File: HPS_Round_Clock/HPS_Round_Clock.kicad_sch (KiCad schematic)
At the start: 113 parts, among them J1 PJ-102AH, J2 Conn_01x06, SW1 Omron_B3F_SPST, SW2 Omron_B3F_SPST, SW3 Omron_B3F_SPST, SW4 Omron_B3F_SPST, SW5 Omron_B3F_SPST, U1 L7805, U2 DS1307_DIP-8, U3 MAX7219, U4 ATmega328-PU, U5 TSOP38238, Y1 Crystal_16MHz, Y2 Crystal_32768Hz

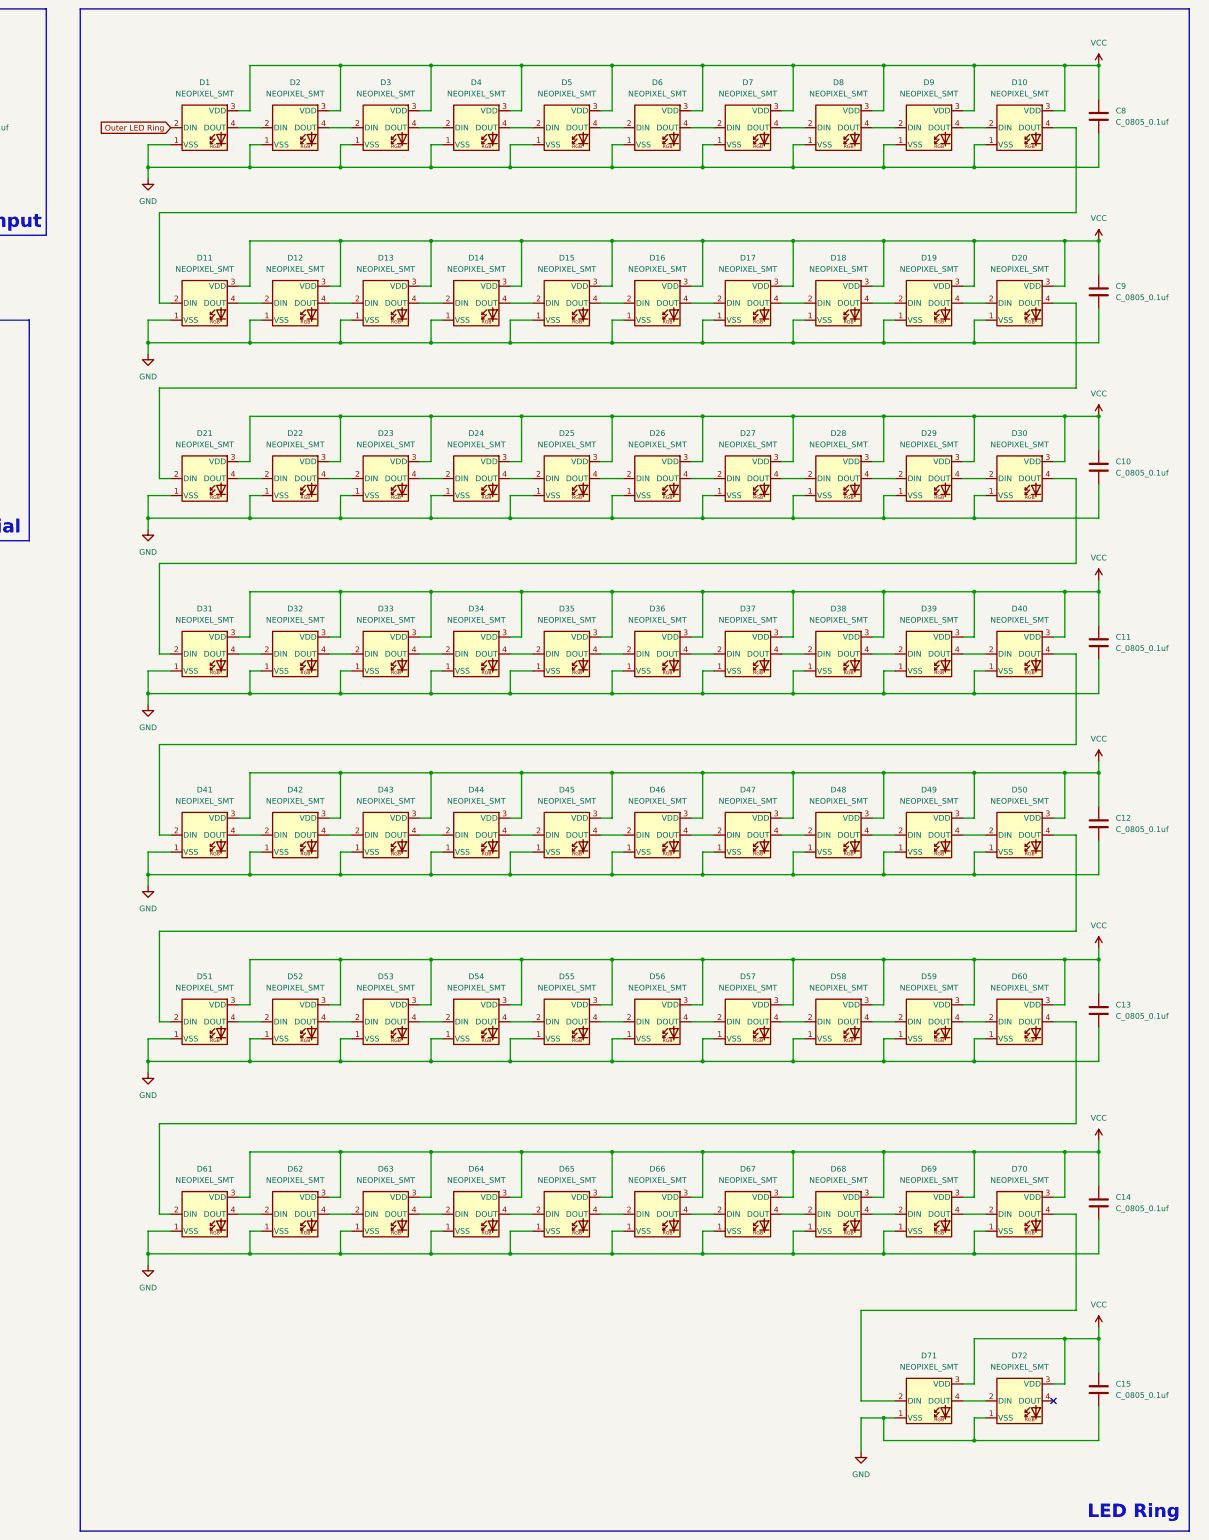
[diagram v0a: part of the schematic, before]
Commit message: Update HPS_Round_Clock.kicad_sch
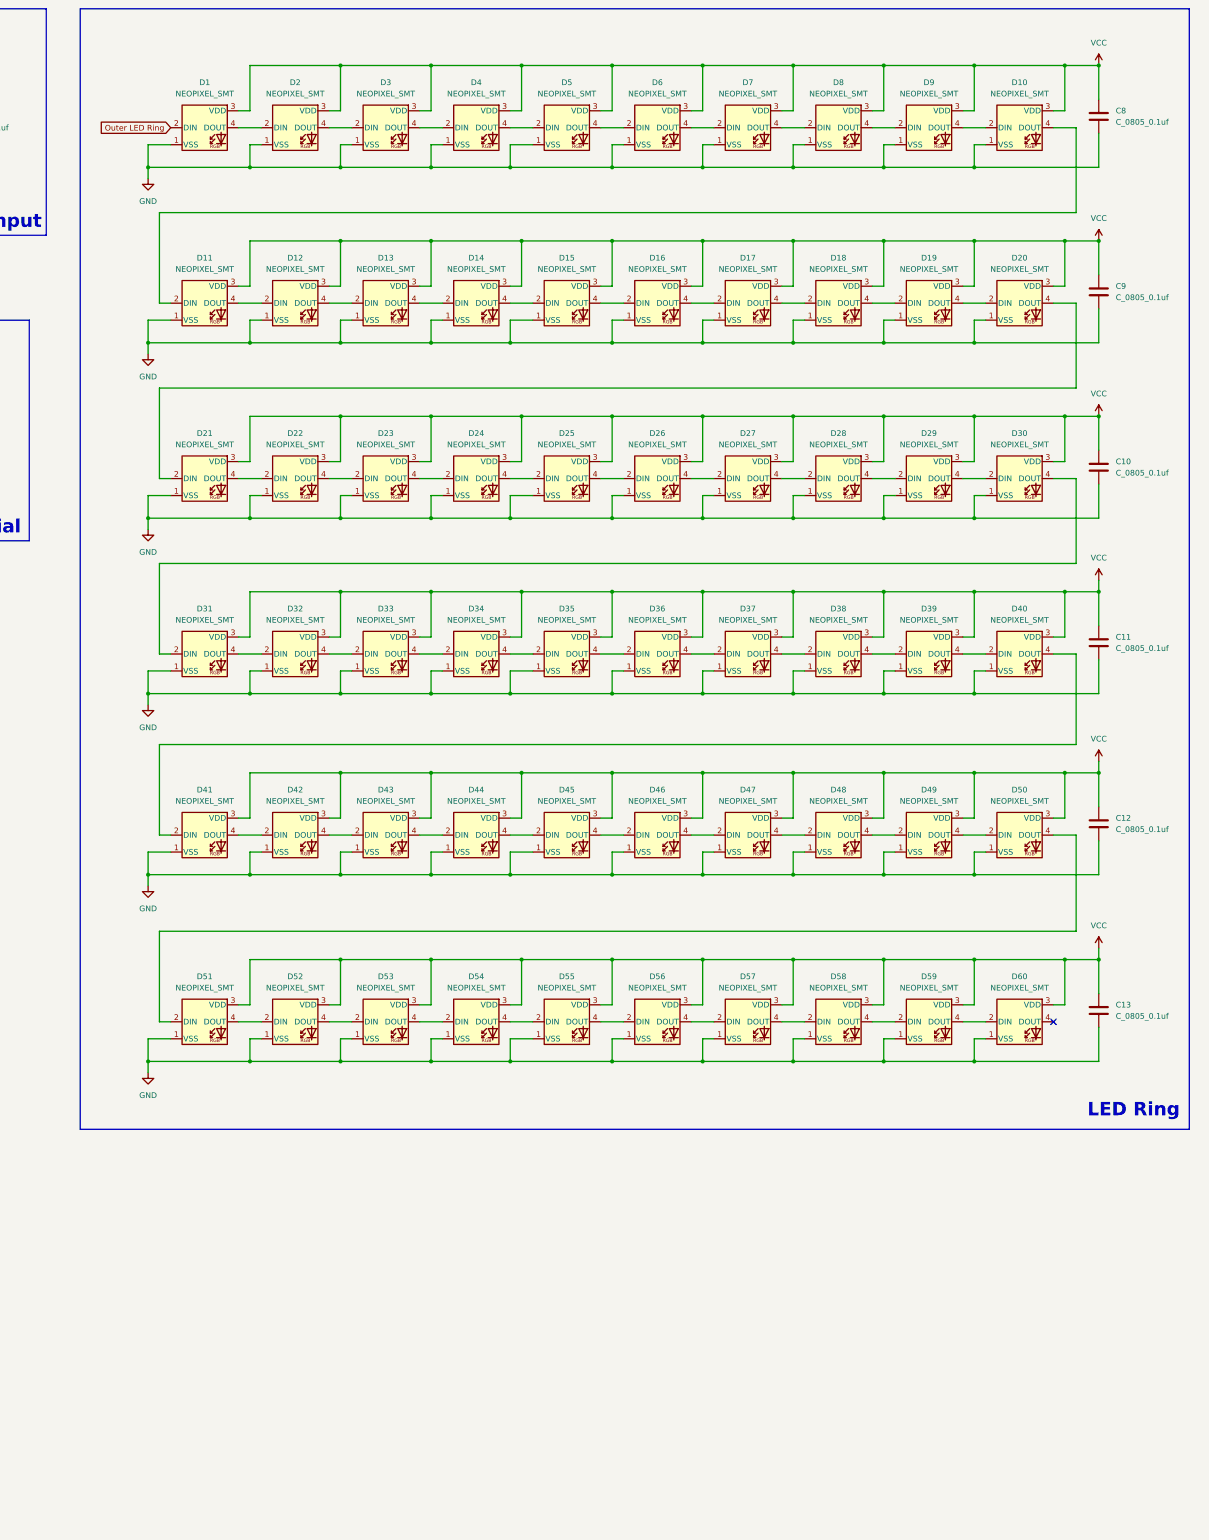
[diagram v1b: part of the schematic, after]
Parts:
- removed C14, C15: C_0805_0.1uf, footprints:C_0805_2012Metric, symbol HPS:C_0805_0.1uf
- removed D61, D62, D63, D64, D65, D66, D67, D68, D69, D70, D71, D72: NEOPIXEL_SMT, footprints:LED_SK6812_PLCC4_5.0x5.0mm_P3.2mm, symbol HPS:NEOPIXEL_SMT
